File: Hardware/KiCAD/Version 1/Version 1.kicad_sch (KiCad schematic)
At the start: 6 parts

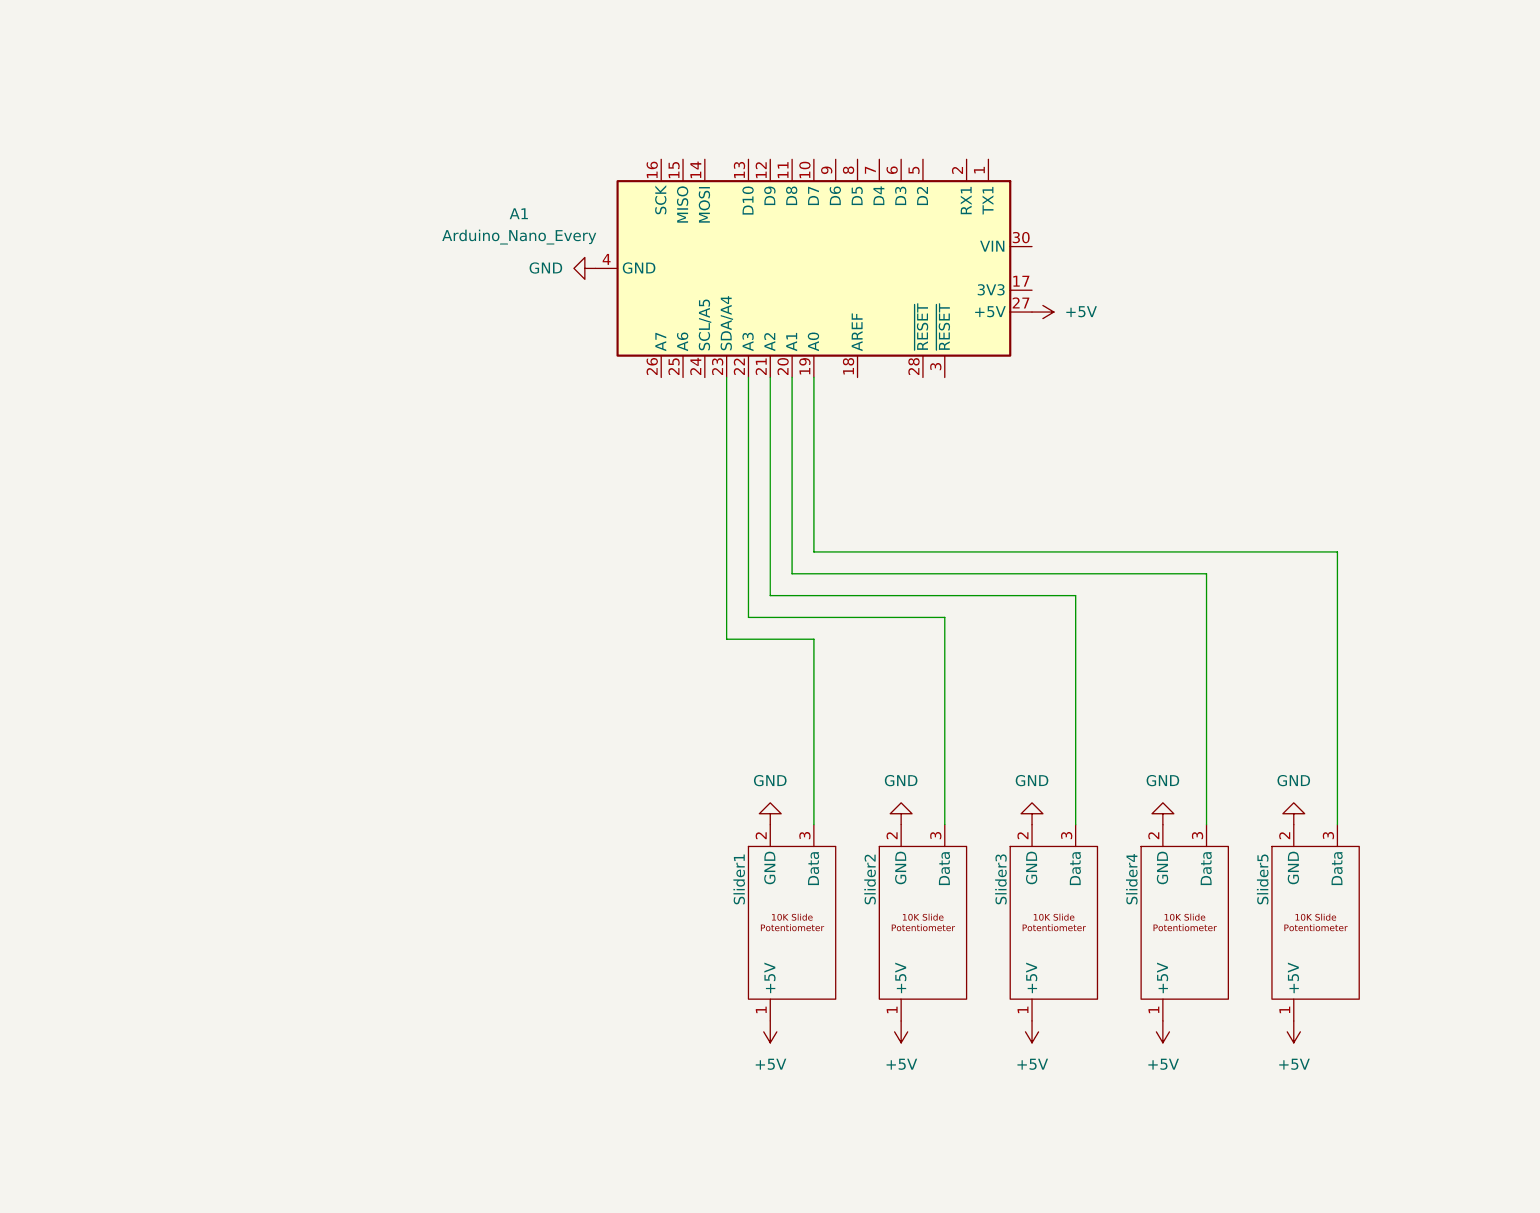
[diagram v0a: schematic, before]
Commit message: pcb progress
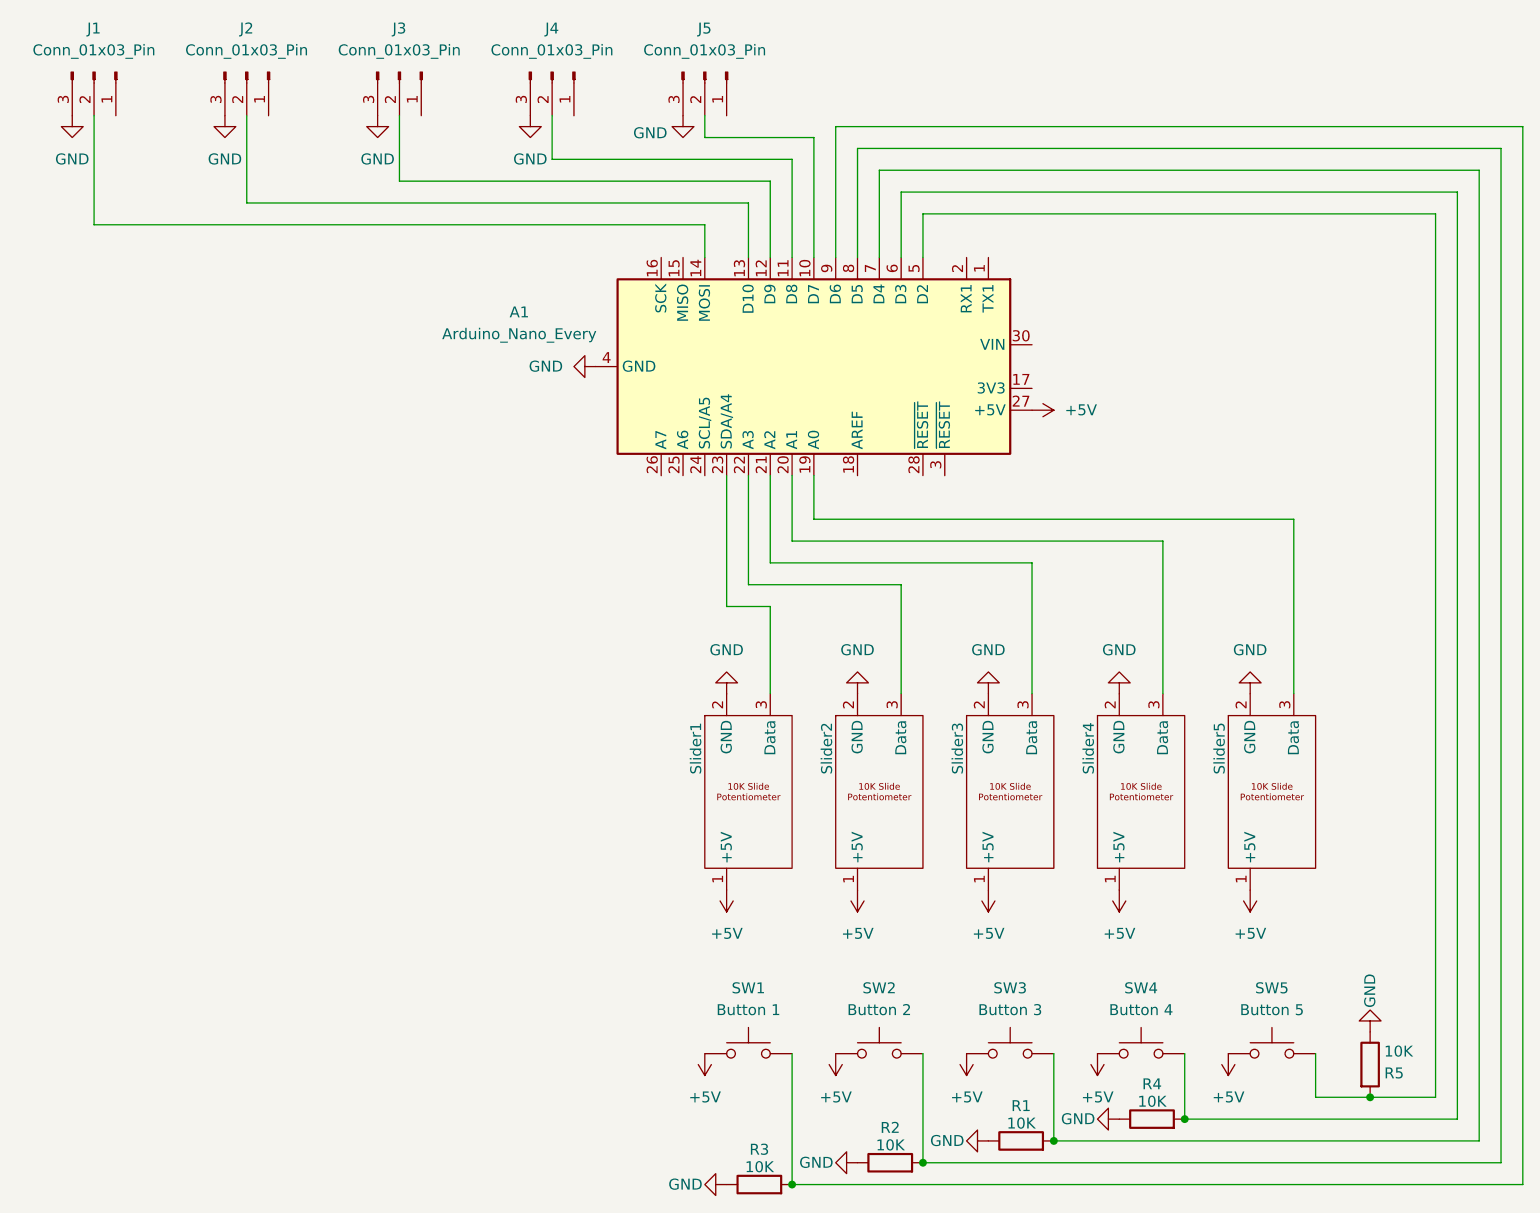
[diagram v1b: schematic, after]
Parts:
- added J1, J2, J3, J4, J5: Conn_01x03_Pin, Connector_PinHeader_2.54mm:PinHeader_1x03_P2.54mm_Vertical, symbol Connector:Conn_01x03_Pin
- added R1, R2, R3, R4, R5: 10K, Resistor_THT:R_Axial_DIN0204_L3.6mm_D1.6mm_P7.62mm_Horizontal, symbol Device:R
- added SW1: Button 1, Button_Switch_Keyboard:SW_Cherry_MX_1.00u_PCB, symbol Switch:SW_Push
- added SW2: Button 2, Button_Switch_Keyboard:SW_Cherry_MX_1.00u_PCB, symbol Switch:SW_Push
- added SW3: Button 3, Button_Switch_Keyboard:SW_Cherry_MX_1.00u_PCB, symbol Switch:SW_Push
- added SW4: Button 4, Button_Switch_Keyboard:SW_Cherry_MX_1.00u_PCB, symbol Switch:SW_Push
- added SW5: Button 5, Button_Switch_Keyboard:SW_Cherry_MX_1.00u_PCB, symbol Switch:SW_Push
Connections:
- net +5V: now also SW1.1, SW2.1, SW3.1, SW4.1, SW5.1
- net GND: now also J1.3 (Pin_3), J2.3 (Pin_3), J3.3 (Pin_3), J4.3 (Pin_3), J5.3 (Pin_3), R1.1, R2.1, R3.1, R4.1, R5.1
- net at A1.10 (D7): now also J5.2 (Pin_2)
- net at A1.11 (D8): now also J4.2 (Pin_2)
- net at A1.12 (D9): now also J3.2 (Pin_2)
- net at A1.13 (D10): now also J2.2 (Pin_2)
- net at A1.14 (MOSI): now also J1.2 (Pin_2)
- net at A1.5 (D2): now also R5.2, SW5.2
- net at A1.6 (D3): now also R4.2, SW4.2
- net at A1.7 (D4): now also R1.2, SW3.2
- net at A1.8 (D5): now also R2.2, SW2.2
- net at A1.9 (D6): now also R3.2, SW1.2
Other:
- moved on the sheet: A1, Slider1, Slider2, Slider3, Slider4, Slider5
